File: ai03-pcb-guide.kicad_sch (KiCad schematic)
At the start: 21 parts, among them J1 Conn_01x04_Socket, J2 AVR-ISP-6, J3 Conn_01x05_Socket, U1 ATmega32U4-A, Y1 16MHz

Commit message: Almost finished
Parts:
- C1, C2, C3, C4, C5, C6, C7, C8: footprint Capacitor_SMD:C_0805_2012Metric -> Capacitor_SMD:C_0603_1608Metric
- R1, R2, R3, R4, R5, R6, R7: footprint Resistor_SMD:R_0805_2012Metric -> Resistor_SMD:R_0603_1608Metric
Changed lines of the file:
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@@
 			)
 		)
-		(property "Footprint" "Resistor_SMD:R_0805_2012Metric"
+		(property "Footprint" "Resistor_SMD:R_0603_1608Metric"
 			(at 39.37 30.48 0)
 			(hide yes)
@@
 			)
 		)
-		(property "Footprint" "Capacitor_SMD:C_0805_2012Metric"
+		(property "Footprint" "Capacitor_SMD:C_0603_1608Metric"
 			(at 33.02 101.6 0)
 			(hide yes)
@@
 			)
 		)
-		(property "Footprint" "Capacitor_SMD:C_0805_2012Metric"
+		(property "Footprint" "Capacitor_SMD:C_0603_1608Metric"
 			(at 69.85 71.12 0)
 			(hide yes)
@@
 			)
 		)
-		(property "Footprint" "Resistor_SMD:R_0805_2012Metric"
+		(property "Footprint" "Resistor_SMD:R_0603_1608Metric"
 			(at 34.29 74.93 0)
 			(hide yes)
@@
 			)
 		)
-		(property "Footprint" "Capacitor_SMD:C_0805_2012Metric"
+		(property "Footprint" "Capacitor_SMD:C_0603_1608Metric"
 			(at 22.86 101.6 0)
 			(hide yes)
@@
 			)
 		)
-		(property "Footprint" "Resistor_SMD:R_0805_2012Metric"
+		(property "Footprint" "Resistor_SMD:R_0603_1608Metric"
 			(at 121.92 88.9 0)
 			(hide yes)
@@
 			)
 		)
-		(property "Footprint" "Capacitor_SMD:C_0805_2012Metric"
+		(property "Footprint" "Capacitor_SMD:C_0603_1608Metric"
 			(at 26.67 45.72 0)
 			(hide yes)
@@
 			)
 		)
-		(property "Footprint" "Capacitor_SMD:C_0805_2012Metric"
+		(property "Footprint" "Capacitor_SMD:C_0603_1608Metric"
 			(at 26.67 50.8 0)
 			(hide yes)
@@
 			)
 		)
-		(property "Footprint" "Capacitor_SMD:C_0805_2012Metric"
+		(property "Footprint" "Capacitor_SMD:C_0603_1608Metric"
 			(at 54.61 101.6 0)
 			(hide yes)
@@
 			)
 		)
-		(property "Footprint" "Resistor_SMD:R_0805_2012Metric"
+		(property "Footprint" "Resistor_SMD:R_0603_1608Metric"
 			(at 55.118 170.18 90)
 			(hide yes)
@@
 			)
 		)
-		(property "Footprint" "Capacitor_SMD:C_0805_2012Metric"
+		(property "Footprint" "Capacitor_SMD:C_0603_1608Metric"
 			(at 43.18 101.6 0)
 			(hide yes)
@@
 			)
 		)
-		(property "Footprint" "Resistor_SMD:R_0805_2012Metric"
+		(property "Footprint" "Resistor_SMD:R_0603_1608Metric"
 			(at 34.29 77.47 0)
 			(hide yes)
@@
 			)
 		)
-		(property "Footprint" "Resistor_SMD:R_0805_2012Metric"
+		(property "Footprint" "Resistor_SMD:R_0603_1608Metric"
 			(at 55.118 185.42 90)
 			(hide yes)
@@
 			)
 		)
-		(property "Footprint" "Capacitor_SMD:C_0805_2012Metric"
+		(property "Footprint" "Capacitor_SMD:C_0603_1608Metric"
 			(at 63.1952 165.1 0)
 			(hide yes)
@@
 			)
 		)
-		(property "Footprint" "Resistor_SMD:R_0805_2012Metric"
+		(property "Footprint" "Resistor_SMD:R_0603_1608Metric"
 			(at 57.658 161.29 90)
 			(hide yes)

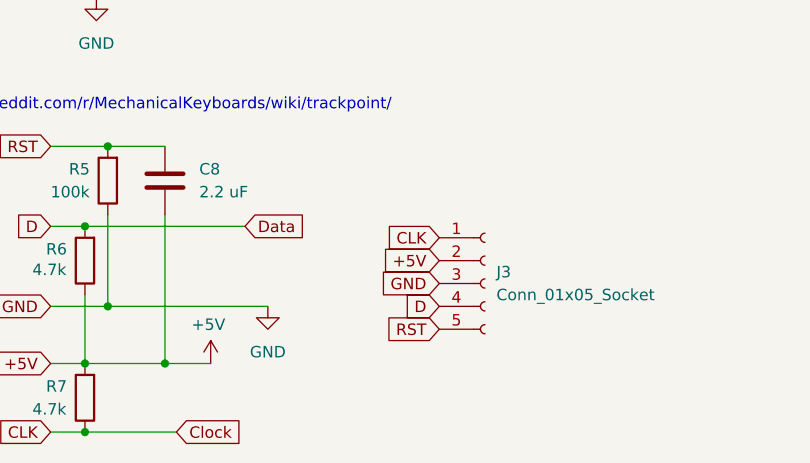
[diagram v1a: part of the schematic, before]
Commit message: Rev 1.0
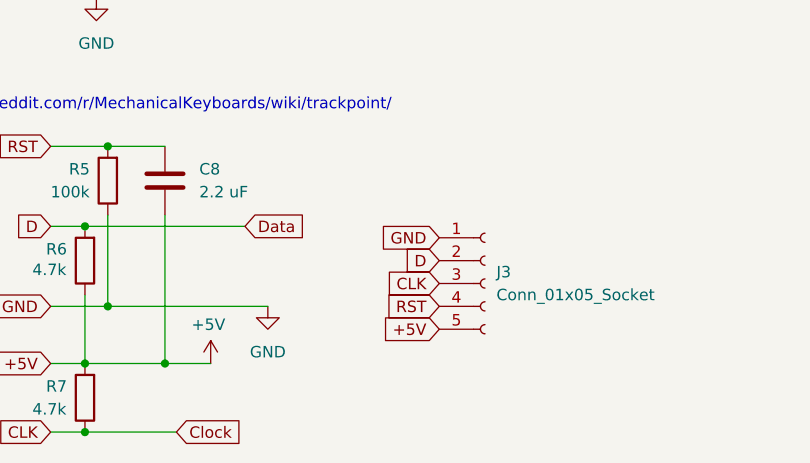
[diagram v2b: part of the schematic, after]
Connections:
- net +5V: now also J3.5 (Pin_5); no longer J3.2 (Pin_2)
- net CLK: now also J3.3 (Pin_3); no longer J3.1 (Pin_1)
- net D: now also J3.2 (Pin_2); no longer J3.4 (Pin_4)
- net GND: now also J3.1 (Pin_1); no longer J3.3 (Pin_3)
- net RST: now also J3.4 (Pin_4); no longer J3.5 (Pin_5)
